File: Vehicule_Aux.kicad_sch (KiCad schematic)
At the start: 16 parts, among them Q43 IRLZ44N, U11 LM339

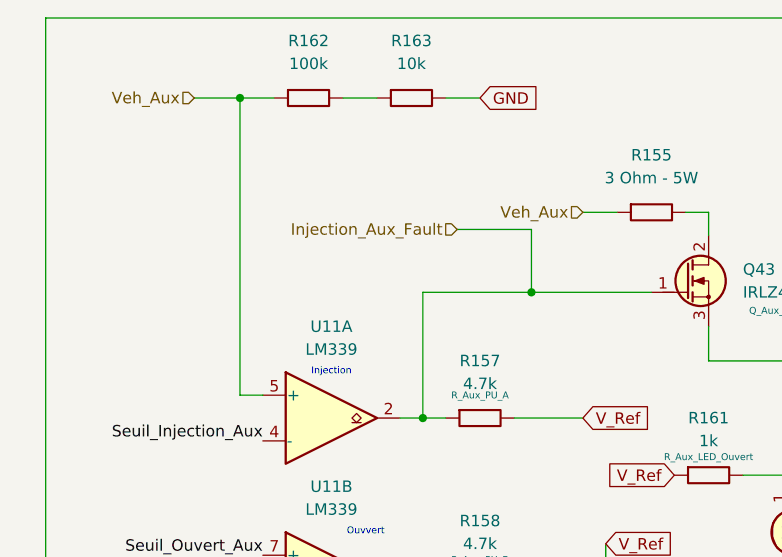
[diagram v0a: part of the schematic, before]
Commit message: Add files via upload
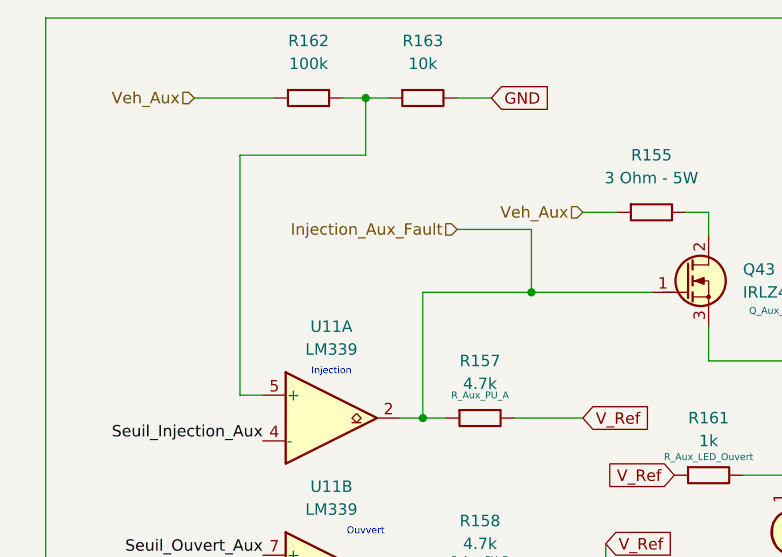
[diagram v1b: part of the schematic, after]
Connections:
- net Veh_Aux: no longer U11.5 (+)
- net at R162.2, R163.1: now also U11.5 (+)
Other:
- moved on the sheet: R163
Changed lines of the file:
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@@
 	)
 	(junction
-		(at 100.33 34.29)
+		(at 114.3 34.29)
 		(diameter 0)
 		(color 0 0 0 0)
@@
 	(wire
 		(pts
-			(xy 100.33 34.29) (xy 104.14 34.29)
+			(xy 95.25 34.29) (xy 104.14 34.29)
 		)
 		(stroke
@@
 	(wire
 		(pts
-			(xy 123.19 34.29) (xy 127 34.29)
+			(xy 124.46 34.29) (xy 128.27 34.29)
 		)
 		(stroke
@@
 	(wire
 		(pts
-			(xy 111.76 34.29) (xy 115.57 34.29)
+			(xy 111.76 34.29) (xy 114.3 34.29)
 		)
 		(stroke
@@
 	(wire
 		(pts
+			(xy 114.3 34.29) (xy 116.84 34.29)
+		)
+		(stroke
+			(width 0)
+			(type default)
+		)
+	)
+	(wire
+		(pts
 			(xy 102.87 90.17) (xy 78.74 90.17)
 		)
@@
 	(wire
 		(pts
+			(xy 114.3 34.29) (xy 114.3 40.64)
+		)
+		(stroke
+			(width 0)
+			(type default)
+		)
+	)
+	(wire
+		(pts
 			(xy 204.47 45.72) (xy 204.47 43.18)
 		)
@@
 	(wire
 		(pts
-			(xy 100.33 67.31) (xy 100.33 34.29)
-		)
-		(stroke
-			(width 0)
-			(type default)
-		)
-	)
-	(wire
-		(pts
-			(xy 95.25 34.29) (xy 100.33 34.29)
-		)
-		(stroke
-			(width 0)
-			(type default)
-		)
-	)
-	(wire
-		(pts
 			(xy 152.4 109.22) (xy 137.16 109.22)
 		)
@@
 	(wire
 		(pts
+			(xy 100.33 40.64) (xy 114.3 40.64)
+		)
+		(stroke
+			(width 0)
+			(type default)
+		)
+	)
+	(wire
+		(pts
 			(xy 152.4 97.79) (xy 152.4 99.06)
 		)
@@
 		(pts
 			(xy 152.4 63.5) (xy 170.18 63.5)
+		)
+		(stroke
+			(width 0)
+			(type default)
+		)
+	)
+	(wire
+		(pts
+			(xy 100.33 67.31) (xy 100.33 40.64)
 		)
 		(stroke
@@
 	(global_label "GND"
 		(shape input)
-		(at 127 34.29 0)
+		(at 128.27 34.29 0)
 		(fields_autoplaced yes)
 		(effects
@@
 		)
 		(property "Intersheetrefs" "${INTERSHEET_REFS}"
-			(at 133.8557 34.29 0)
+			(at 135.1257 34.29 0)
 			(hide yes)
 			(show_name no)
@@
 	(symbol
 		(lib_id "PCM_SL_Resistors:10k")
-		(at 119.38 34.29 0)
+		(at 120.65 34.29 0)
 		(unit 1)
 		(body_style 1)
@@
 		(fields_autoplaced yes)
 		(property "Reference" "R163"
-			(at 119.38 27.94 0)
+			(at 120.65 27.94 0)
 			(show_name no)
 			(do_not_autoplace no)
@@
 		)
 		(property "Value" "10k"
-			(at 119.38 30.48 0)
+			(at 120.65 30.48 0)
 			(show_name no)
 			(do_not_autoplace no)
@@
 		)
 		(property "Footprint" "Resistor_THT:R_Axial_DIN0207_L6.3mm_D2.5mm_P10.16mm_Horizontal"
-			(at 120.269 38.608 0)
+			(at 121.539 38.608 0)
 			(hide yes)
 			(show_name no)
@@
 		)
 		(property "Datasheet" ""
-			(at 119.888 34.29 0)
+			(at 121.158 34.29 0)
 			(hide yes)
 			(show_name no)
@@
 		)
 		(property "Description" "10kΩ, 1/4W Resistor"
-			(at 119.38 34.29 0)
-			(hide yes)
-			(show_name no)
+			(at 120.65 34.29 0)
+			(hide yes)
+			(show_name no)
